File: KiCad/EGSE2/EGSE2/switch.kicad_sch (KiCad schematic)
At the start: 7 parts, among them Q1 SIS412DN-T1-GE3, Q2 SIS412DN-T1-GE3, Q3 SIS412DN-T1-GE3, Q4 SIS412DN-T1-GE3

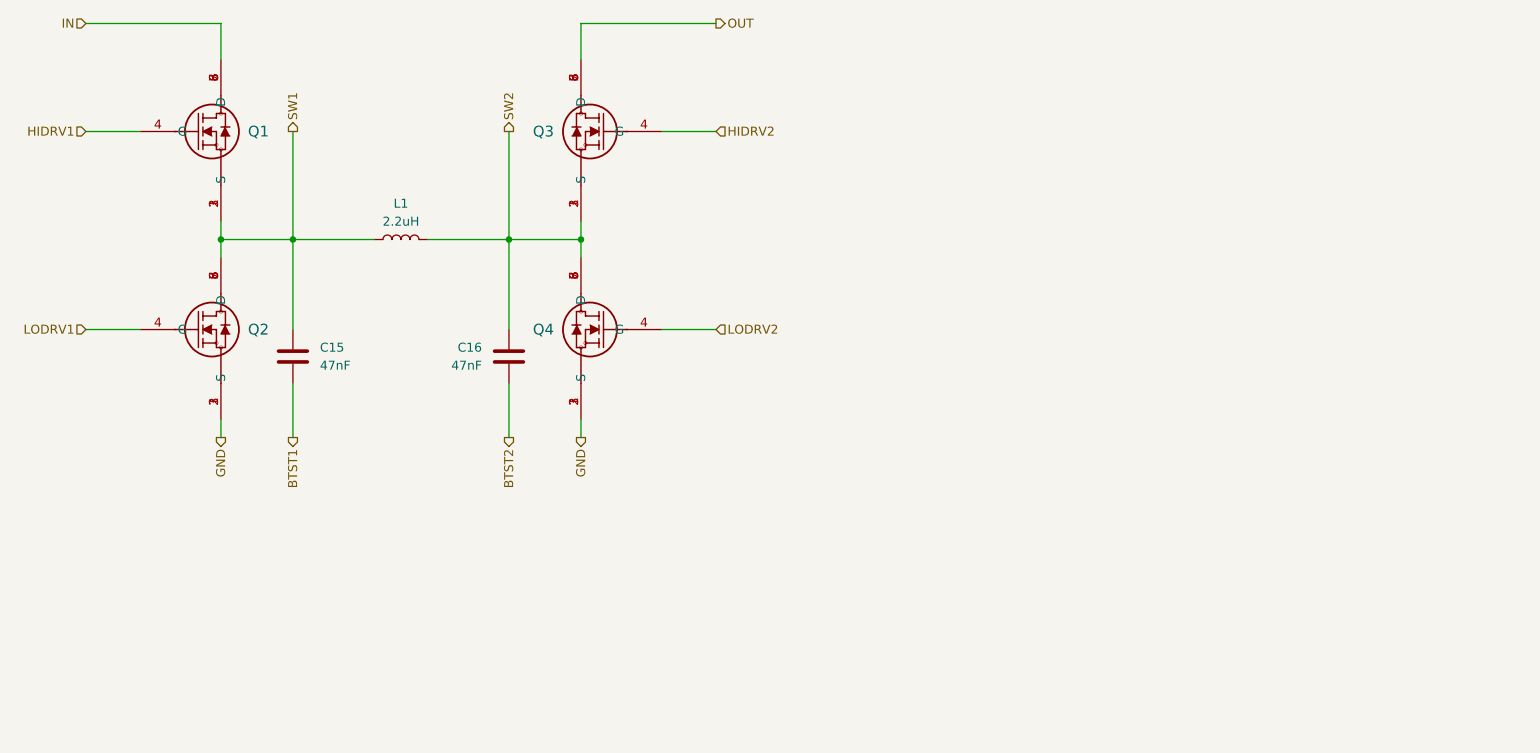
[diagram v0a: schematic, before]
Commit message: gamig on this EGSE type hsi
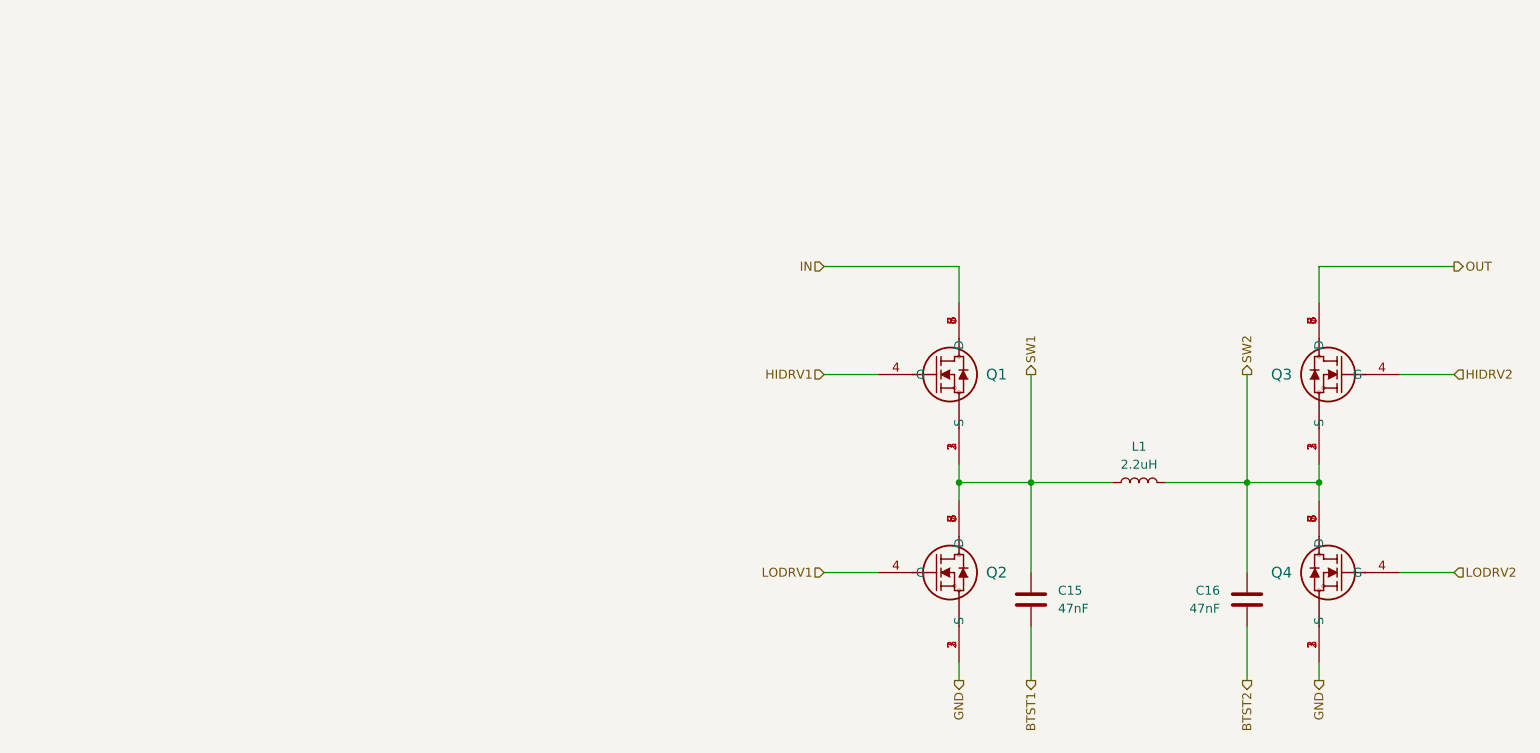
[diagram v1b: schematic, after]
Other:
- moved on the sheet: C15, C16, L1, Q1, Q2, Q3, Q4
